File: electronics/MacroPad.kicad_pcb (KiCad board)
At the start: 2 copper layers, 143.5 x 20.3 mm, 6 parts, among them SW1 SW_Push, SW2 SW_Coded, SW3 SW_Push, SW4 SW_Push, SW5 SW_Push, U1 ProMicro

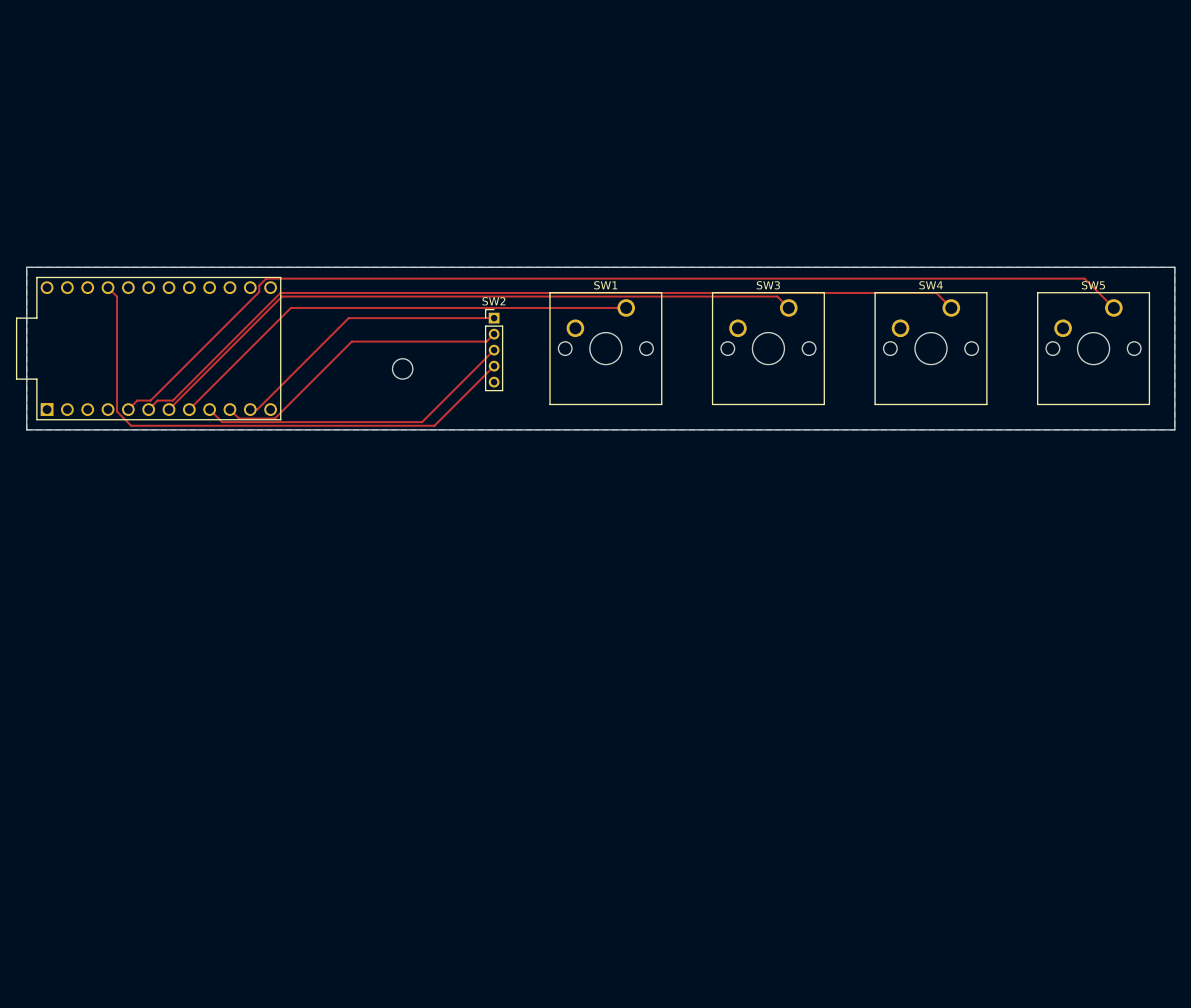
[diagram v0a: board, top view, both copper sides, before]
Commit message: cleaned for v2
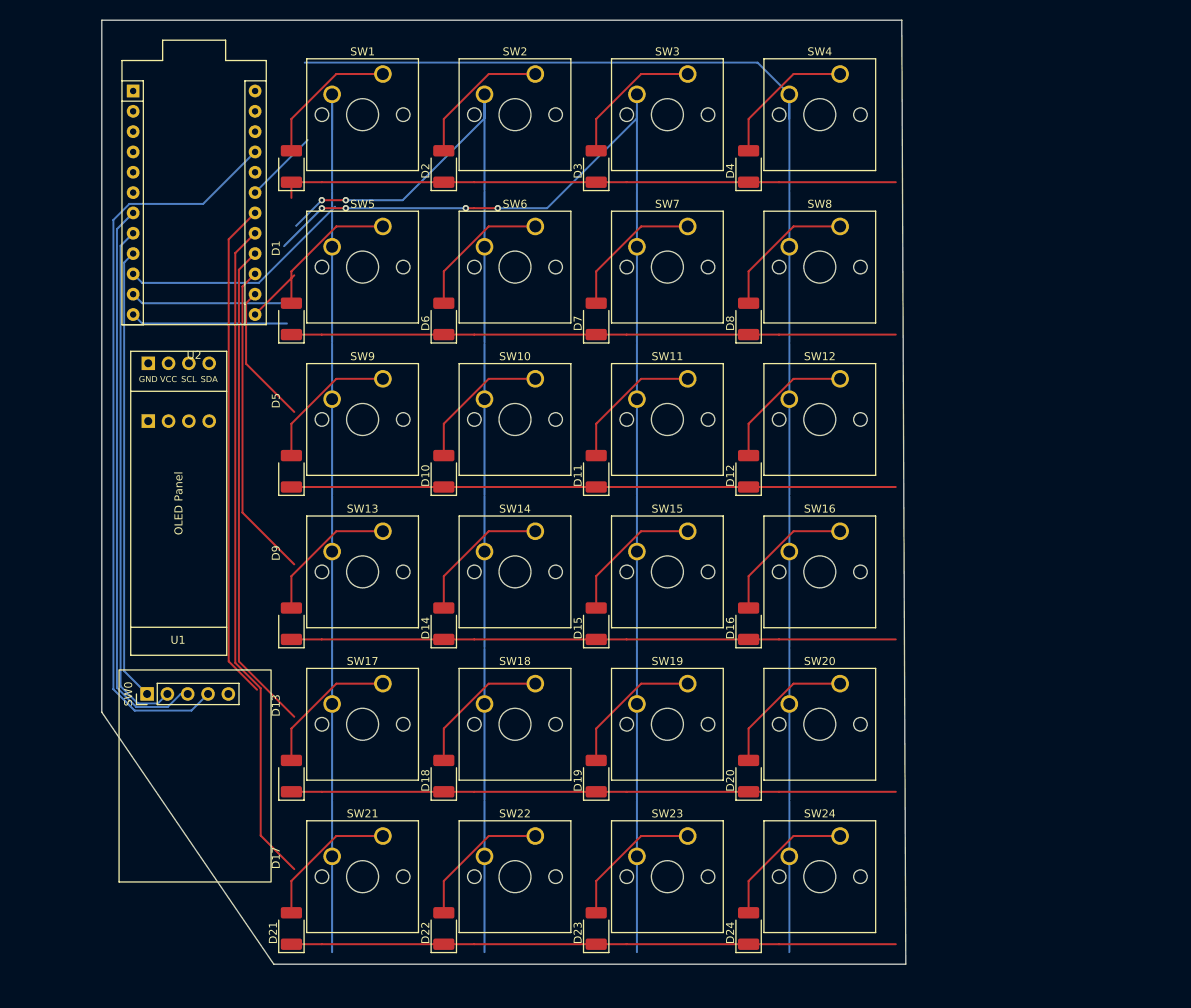
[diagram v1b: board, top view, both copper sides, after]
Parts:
- added D1: 1N4148, Diode_SMD:D_1210_3225Metric_Pad1.42x2.65mm_HandSolder, F.Cu at (104.2, 60.3)
- added D10: 1N4148, Diode_SMD:D_1210_3225Metric_Pad1.42x2.65mm_HandSolder, F.Cu at (123.2, 98.4)
- added D11: 1N4148, Diode_SMD:D_1210_3225Metric_Pad1.42x2.65mm_HandSolder, F.Cu at (142.3, 98.4)
- added D12: 1N4148, Diode_SMD:D_1210_3225Metric_Pad1.42x2.65mm_HandSolder, F.Cu at (161.3, 98.4)
- added D13: 1N4148, Diode_SMD:D_1210_3225Metric_Pad1.42x2.65mm_HandSolder, F.Cu at (104.2, 117.5)
- added D14: 1N4148, Diode_SMD:D_1210_3225Metric_Pad1.42x2.65mm_HandSolder, F.Cu at (123.2, 117.5)
- added D15: 1N4148, Diode_SMD:D_1210_3225Metric_Pad1.42x2.65mm_HandSolder, F.Cu at (142.3, 117.5)
- added D16: 1N4148, Diode_SMD:D_1210_3225Metric_Pad1.42x2.65mm_HandSolder, F.Cu at (161.3, 117.5)
- added D17: 1N4148, Diode_SMD:D_1210_3225Metric_Pad1.42x2.65mm_HandSolder, F.Cu at (104.2, 136.5)
- added D18: 1N4148, Diode_SMD:D_1210_3225Metric_Pad1.42x2.65mm_HandSolder, F.Cu at (123.2, 136.5)
- added D19: 1N4148, Diode_SMD:D_1210_3225Metric_Pad1.42x2.65mm_HandSolder, F.Cu at (142.3, 136.5)
- added D2: 1N4148, Diode_SMD:D_1210_3225Metric_Pad1.42x2.65mm_HandSolder, F.Cu at (123.2, 60.3)
- added D20: 1N4148, Diode_SMD:D_1210_3225Metric_Pad1.42x2.65mm_HandSolder, F.Cu at (161.3, 136.5)
- added D21: 1N4148, Diode_SMD:D_1210_3225Metric_Pad1.42x2.65mm_HandSolder, F.Cu at (104.2, 155.6)
- added D22: 1N4148, Diode_SMD:D_1210_3225Metric_Pad1.42x2.65mm_HandSolder, F.Cu at (123.2, 155.6)
- added D23: 1N4148, Diode_SMD:D_1210_3225Metric_Pad1.42x2.65mm_HandSolder, F.Cu at (142.3, 155.6)
- added D24: 1N4148, Diode_SMD:D_1210_3225Metric_Pad1.42x2.65mm_HandSolder, F.Cu at (161.3, 155.6)
- added D3: 1N4148, Diode_SMD:D_1210_3225Metric_Pad1.42x2.65mm_HandSolder, F.Cu at (142.3, 60.3)
- added D4: 1N4148, Diode_SMD:D_1210_3225Metric_Pad1.42x2.65mm_HandSolder, F.Cu at (161.3, 60.3)
- added D5: 1N4148, Diode_SMD:D_1210_3225Metric_Pad1.42x2.65mm_HandSolder, F.Cu at (104.2, 79.4)
- added D6: 1N4148, Diode_SMD:D_1210_3225Metric_Pad1.42x2.65mm_HandSolder, F.Cu at (123.2, 79.4)
- added D7: 1N4148, Diode_SMD:D_1210_3225Metric_Pad1.42x2.65mm_HandSolder, F.Cu at (142.3, 79.4)
- added D8: 1N4148, Diode_SMD:D_1210_3225Metric_Pad1.42x2.65mm_HandSolder, F.Cu at (161.3, 79.4)
- added D9: 1N4148, Diode_SMD:D_1210_3225Metric_Pad1.42x2.65mm_HandSolder, F.Cu at (104.2, 98.4)
- added SW0: SW_Coded, Connector_PinHeader_2.54mm:PinHeader_1x05_P2.54mm_Vertical, F.Cu at (86.2, 125.7)
- added SW10: SW_Push, proj_components:SW_Cherry_MX_1.00u_PCB, F.Cu at (134.7, 86.3)
- added SW11: SW_Push, proj_components:SW_Cherry_MX_1.00u_PCB, F.Cu at (153.7, 86.3)
- added SW12: SW_Push, proj_components:SW_Cherry_MX_1.00u_PCB, F.Cu at (172.8, 86.3)
- added SW13: SW_Push, proj_components:SW_Cherry_MX_1.00u_PCB, F.Cu at (115.6, 105.4)
- added SW14: SW_Push, proj_components:SW_Cherry_MX_1.00u_PCB, F.Cu at (134.7, 105.4)
- added SW15: SW_Push, proj_components:SW_Cherry_MX_1.00u_PCB, F.Cu at (153.7, 105.4)
- added SW16: SW_Push, proj_components:SW_Cherry_MX_1.00u_PCB, F.Cu at (172.8, 105.4)
- added SW17: SW_Push, proj_components:SW_Cherry_MX_1.00u_PCB, F.Cu at (115.6, 124.4)
- added SW18: SW_Push, proj_components:SW_Cherry_MX_1.00u_PCB, F.Cu at (134.7, 124.4)
- added SW19: SW_Push, proj_components:SW_Cherry_MX_1.00u_PCB, F.Cu at (153.7, 124.4)
- added SW20: SW_Push, proj_components:SW_Cherry_MX_1.00u_PCB, F.Cu at (172.8, 124.4)
- added SW21: SW_Push, proj_components:SW_Cherry_MX_1.00u_PCB, F.Cu at (115.6, 143.5)
- added SW22: SW_Push, proj_components:SW_Cherry_MX_1.00u_PCB, F.Cu at (134.7, 143.5)
- added SW23: SW_Push, proj_components:SW_Cherry_MX_1.00u_PCB, F.Cu at (153.7, 143.5)
- added SW24: SW_Push, proj_components:SW_Cherry_MX_1.00u_PCB, F.Cu at (172.8, 143.5)
- added SW6: SW_Push, proj_components:SW_Cherry_MX_1.00u_PCB, F.Cu at (134.7, 67.3)
- added SW7: SW_Push, proj_components:SW_Cherry_MX_1.00u_PCB, F.Cu at (153.7, 67.3)
- added SW8: SW_Push, proj_components:SW_Cherry_MX_1.00u_PCB, F.Cu at (172.8, 67.3)
- added SW9: SW_Push, proj_components:SW_Cherry_MX_1.00u_PCB, F.Cu at (115.6, 86.3)
- added U2: ProMicro, proj_components:Sparkfun_Pro_Micro, F.Cu at (99.7, 78.3)
- added U3: SSD1306, proj_components:SSD1306-0.91-OLED-4pin-128x32, B.Cu at (84.1, 55.1)
- SW1, SW3, SW4, SW5: footprint Button_Switch_Keyboard:SW_Cherry_MX_1.00u_PCB -> proj_components:SW_Cherry_MX_1.00u_PCB
- SW2: value SW_Coded -> SW_Push; footprint Connector_PinHeader_2.00mm:PinHeader_1x05_P2.00mm_Vertical -> proj_components:SW_Cherry_MX_1.00u_PCB
- U1: value ProMicro -> SSD1306; footprint Arduino_Pro_Micro:ProMicro -> proj_components:SSD1306-0.91-OLED-4pin-128x32
- moved SW5 91.9 mm to (115.6, 67.3)
- moved SW1 42.2 mm to (115.6, 48.2)
- moved U1 38.5 mm to (84.1, 120.9), turned to 90 degrees
- moved SW4 32.4 mm to (172.8, 48.2)
- moved SW3 31.9 mm to (153.7, 48.2)
- moved SW2 30.9 mm to (134.7, 48.2)
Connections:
- SW1 pad 1: Net-(SW1-Pad1) -> Net-(D1-A)
- SW1 pad 2: GND -> IN1
- SW2 pad 1: Net-(SW2-Pad1) -> Net-(D2-A)
- SW2 pad 2: Net-(SW2-Pad2) -> IN2
- SW3 pad 1: Net-(SW3-Pad1) -> Net-(D3-A)
- SW3 pad 2: GND -> IN3
- SW4 pad 1: Net-(SW4-Pad1) -> Net-(D4-A)
- SW4 pad 2: GND -> IN4
- SW5 pad 1: Net-(SW5-Pad1) -> Net-(D5-A)
- SW5 pad 2: GND -> IN1
- U1 pad 1: Net-(U1-Pad1) -> unconnected-(U1-C2P-Pad1)
- U1 pad 2: Net-(U1-Pad2) -> unconnected-(U1-C2N-Pad2)
- U1 pad 3: Net-(U1-Pad3) -> unconnected-(U1-C1P-Pad3)
- U1 pad 4: Net-(U1-Pad4) -> unconnected-(U1-C1N-Pad4)
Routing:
- net IN4: track 0.00 -> 180.9 mm
- net IN3: track 0.00 -> 178.9 mm, vias 0 -> 4
- net IN2: track 0.00 -> 159.7 mm, vias 0 -> 2
- net OUT5: track 0.00 -> 157.2 mm
- net IN1: track 0.00 -> 140.4 mm
- net OUT6: track 0.00 -> 136.0 mm
- net OUT4: track 0.00 -> 135.2 mm
- net Net-(SW5-Pad1): track 131.9 -> 0.00 mm
- net OUT3: track 0.00 -> 113.2 mm
- net Net-(SW4-Pad1): track 107.1 -> 0.00 mm
- net OUT2: track 0.00 -> 91.3 mm
- net Net-(SW3-Pad1): track 83.9 -> 0.00 mm
- net OUT1: track 0.00 -> 82.5 mm
- net SW: track 0.00 -> 70.7 mm
- net DT: track 0.00 -> 64.5 mm
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- removed copper zone on B.Cu, net GND
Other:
- board size 143.5 x 20.3 mm -> 100.5 x 118 mm
- net class Default removed
- board text removed: "MacroPad Jonathan"

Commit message: platformio conversion
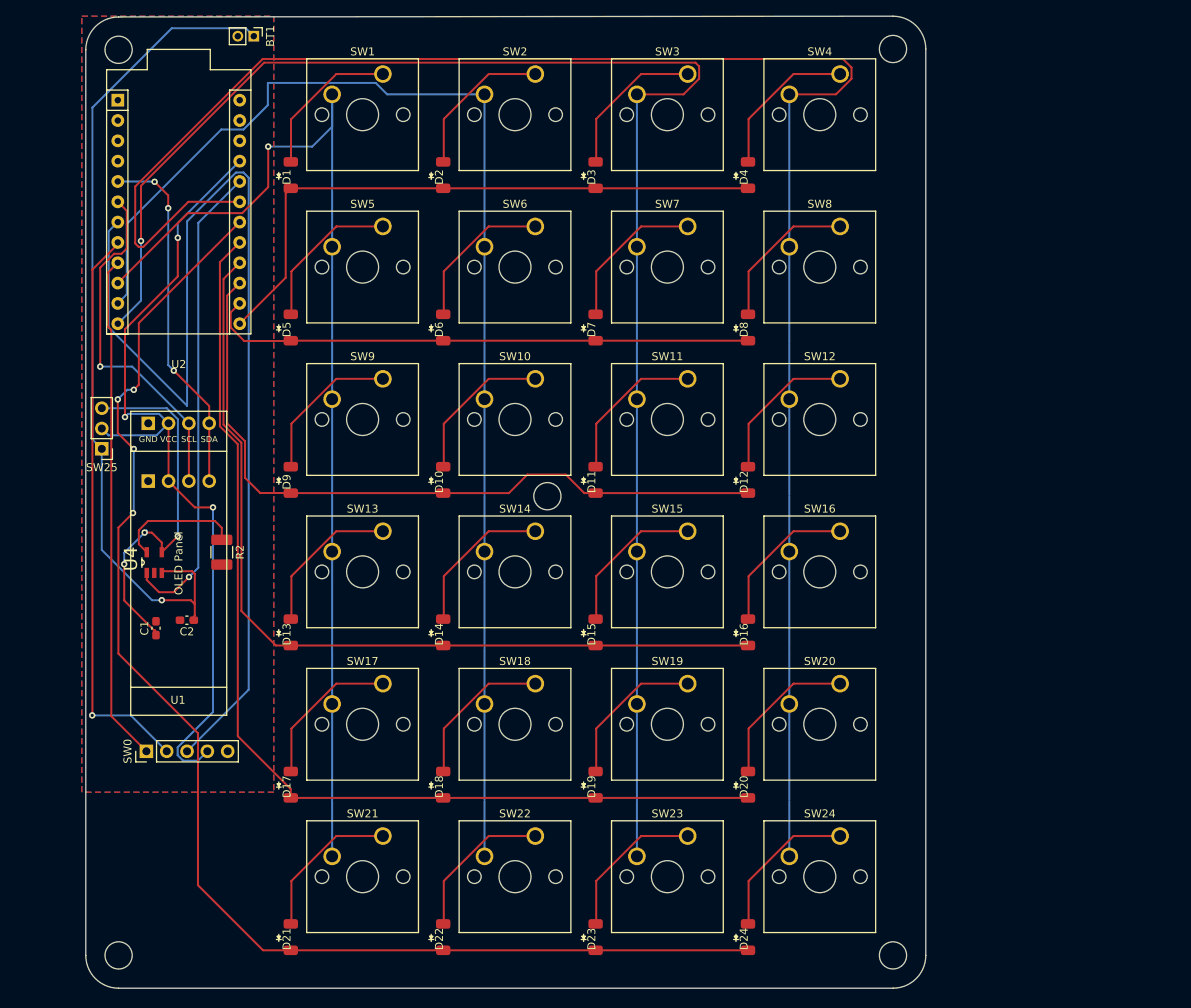
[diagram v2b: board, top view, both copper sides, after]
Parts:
- added BT1: Battery, Connector_PinHeader_2.00mm:PinHeader_1x02_P2.00mm_Vertical, F.Cu at (99.5, 43.5)
- added C1: 4.7uF, Capacitor_SMD:C_0603_1608Metric_Pad1.08x0.95mm_HandSolder, F.Cu at (87.3, 117.5)
- added C2: 4.7uF, Capacitor_SMD:C_0603_1608Metric_Pad1.08x0.95mm_HandSolder, F.Cu at (91.1, 116.5)
- added R2: 2K, Resistor_SMD:R_1210_3225Metric_Pad1.30x2.65mm_HandSolder, F.Cu at (95.5, 108.0)
- added SW25: SW_SPDT, Connector_PinHeader_2.54mm:PinHeader_1x03_P2.54mm_Vertical, F.Cu at (80.5, 95.1)
- added U4: MCP73831T-2ACI_OT, proj_components:SOT95P280X145-5N, F.Cu at (87.1, 109.3)
- D1, D10, D11, D12, D13, D14, D15, D16, D17, D18, D19, D2, D20, D21, D22, D23, D24, D3, D4, D5, D6, D7, D8, D9: value 1N4148 -> LL4148; footprint Diode_SMD:D_1210_3225Metric_Pad1.42x2.65mm_HandSolder -> LL4148:LL4148
- moved U3 7.50 mm to (84.1, 62.6)
- moved U1 7.50 mm to (84.1, 128.4)
- moved SW0 7.17 mm to (86.1, 132.9)
- moved U2 2.24 mm to (97.7, 79.4)
- moved D15 0.51 mm to (142.1, 118.0)
- moved D13 0.51 mm to (104.0, 118.0)
- moved D14 0.51 mm to (123.1, 118.0)
- moved D3 0.51 mm to (142.1, 60.8)
- moved D16 0.51 mm to (161.2, 118.0)
- moved D1 0.51 mm to (104.0, 60.8)
- moved D2 0.51 mm to (123.1, 60.8)
- moved D11 0.51 mm to (142.1, 98.9)
- moved D19 0.51 mm to (142.1, 137.0)
- moved D23 0.51 mm to (142.1, 156.1)
- moved D7 0.51 mm to (142.1, 79.9)
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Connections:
- U2 pad 20: unconnected-(U2-D21/A3/PF4-Pad20) -> STAT
- U2 pad 24: +5V -> unconnected-(U2-RAW-Pad24)
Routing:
- net Net-(BT1-+): track 0.00 -> 105.3 mm, vias 0 -> 1
- net SW: track 70.7 -> 135.9 mm
- net STAT: track 0.00 -> 59.6 mm, vias 0 -> 1
- net Net-(SW25-C): track 0.00 -> 47.4 mm, vias 0 -> 3
- net SDA: track 0.00 -> 44.9 mm, vias 0 -> 3
- net SCL: track 0.00 -> 44.2 mm, vias 0 -> 1
- net IN4: track 180.9 -> 223.8 mm
- net OUT6: track 136.0 -> 167.5 mm, vias 0 -> 4
- net OUT5: track 157.2 -> 131.3 mm
- net OUT4: track 135.2 -> 110.4 mm
- net OUT2: track 91.3 -> 68.8 mm
- net OUT3: track 113.2 -> 91.5 mm
- net IN3: track 178.9 -> 199.5 mm, vias 4 -> 1
- net Net-(U4-PROG): track 0.00 -> 15.9 mm
- net +5V: track 93.7 -> 104.8 mm, vias 0 -> 3
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- added copper zone on B.Cu, net GND
- added copper zone on F.Cu, net GND
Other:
- board size 100.5 x 118 mm -> 105 x 121.5 mm
- board text added: "macropad 6/19/24"

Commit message: update docs
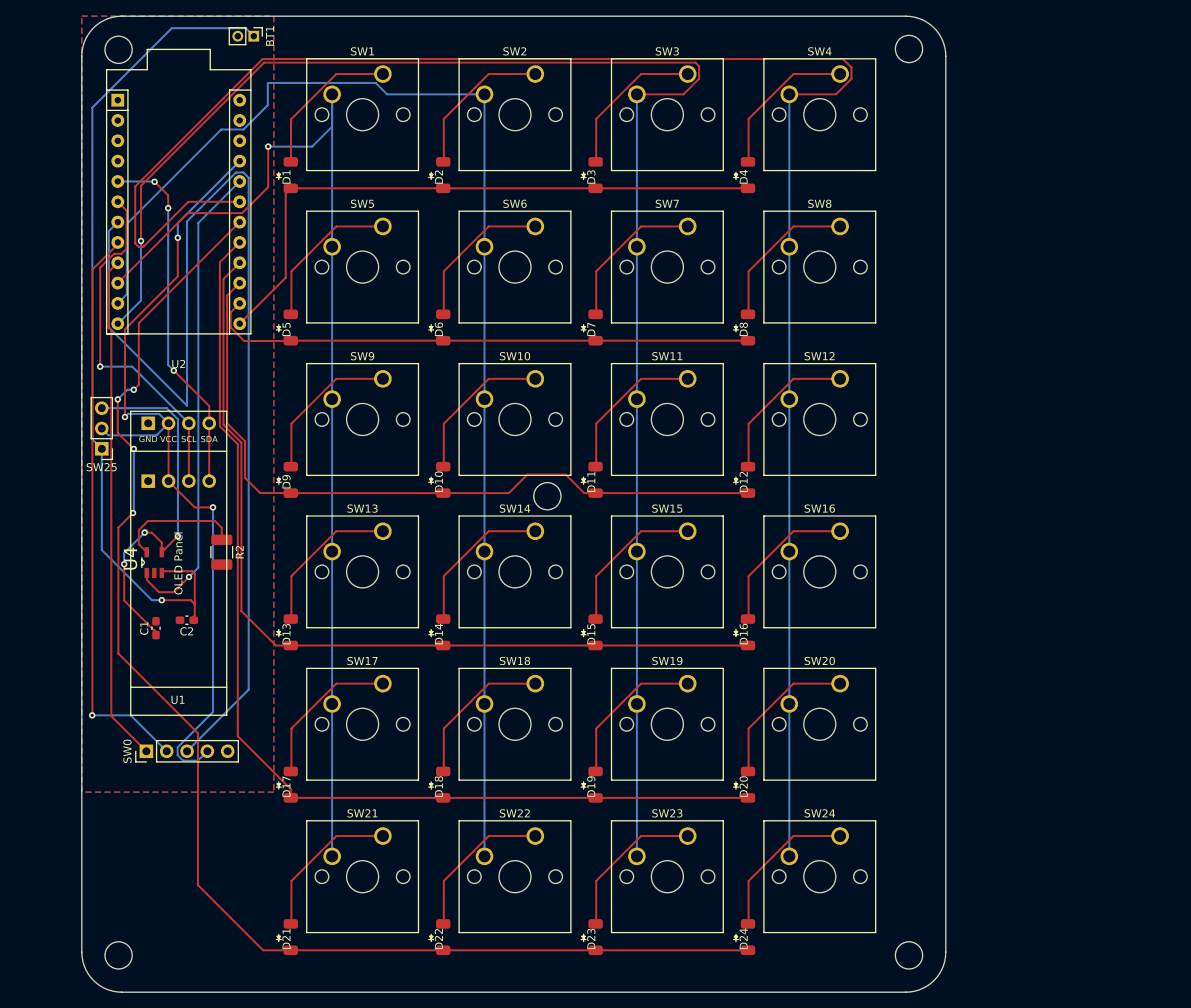
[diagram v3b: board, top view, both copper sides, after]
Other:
- board size 105 x 121.5 mm -> 108 x 122 mm
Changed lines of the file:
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@@
 	)
 	(gr_line
-		(start 179.4 41)
-		(end 82.599138 41.099138)
+		(start 83 41)
+		(end 181 41)
 		(stroke
 			(width 0.05)
@@
 		(layer "Edge.Cuts")
 	)
-	(gr_arc
-		(start 179.4 41)
-		(mid 182.299138 42.200862)
-		(end 183.5 45.1)
+	(gr_line
+		(start 78 158)
+		(end 78 46)
+		(stroke
+			(width 0.05)
+			(type default)
+		)
+		(layer "Edge.Cuts")
+	)
+	(gr_line
+		(start 181 163)
+		(end 83 163)
 		(stroke
 			(width 0.05)
@@
 	)
 	(gr_line
-		(start 78.499138 45.199138)
-		(end 78.499138 158.400862)
+		(start 186 46)
+		(end 186 158)
 		(stroke
 			(width 0.05)
@@
 		(layer "Edge.Cuts")
 	)
+	(gr_arc
+		(start 78 46)
+		(mid 79.464466 42.464466)
+		(end 83 41)
+		(stroke
+			(width 0.05)
+			(type default)
+		)
+		(layer "Edge.Cuts")
+	)
 	(gr_circle
-		(center 179.4 158.4)
-		(end 177.7 158.4)
+		(center 181.4 158.4)
+		(end 179.7 158.4)
 		(stroke
 			(width 0.05)
@@
 		)
 		(fill none)
-		(layer "Edge.Cuts")
-	)
-	(gr_arc
-		(start 82.599138 162.500862)
-		(mid 79.7 161.3)
-		(end 78.499138 158.400862)
-		(stroke
-			(width 0.05)
-			(type default)
-		)
 		(layer "Edge.Cuts")
 	)
@@
 		(layer "Edge.Cuts")
 	)
-	(gr_line
-		(start 183.5 158.4)
-		(end 183.5 45.1)
+	(gr_arc
+		(start 181 41)
+		(mid 184.535534 42.464466)
+		(end 186 46)
 		(stroke
 			(width 0.05)
@@
 		(layer "Edge.Cuts")
 	)
-	(gr_line
-		(start 82.599138 162.500862)
-		(end 179.4 162.5)
-		(stroke
-			(width 0.05)
-			(type default)
-		)
-		(layer "Edge.Cuts")
-	)
 	(gr_arc
-		(start 78.499138 45.199138)
-		(mid 79.7 42.3)
-		(end 82.599138 41.099138)
+		(start 83 163)
+		(mid 79.464466 161.535534)
+		(end 78 158)
 		(stroke
 			(width 0.05)
@@
 	)
 	(gr_arc
-		(start 183.5 158.4)
-		(mid 182.299138 161.299138)
-		(end 179.4 162.5)
+		(start 186 158)
+		(mid 184.535534 161.535534)
+		(end 181 163)
 		(stroke
 			(width 0.05)
@@
 	)
 	(gr_circle
-		(center 179.4 45.1)
-		(end 179.4 46.8)
+		(center 181.4 45.1)
+		(end 181.4 46.8)
 		(stroke
 			(width 0.05)
@@
 		(net 1)
 		(net_name "GND")
+		(locked yes)
 		(layers "F&B.Cu")
 		(name "gnd")
